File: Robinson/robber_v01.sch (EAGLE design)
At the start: 35 parts, among them J1 3.7_LIPO, J2 3.3-4.5 Motor, Q1 DMP1045U, Q2 MMBT2222A, U2 MCP73831

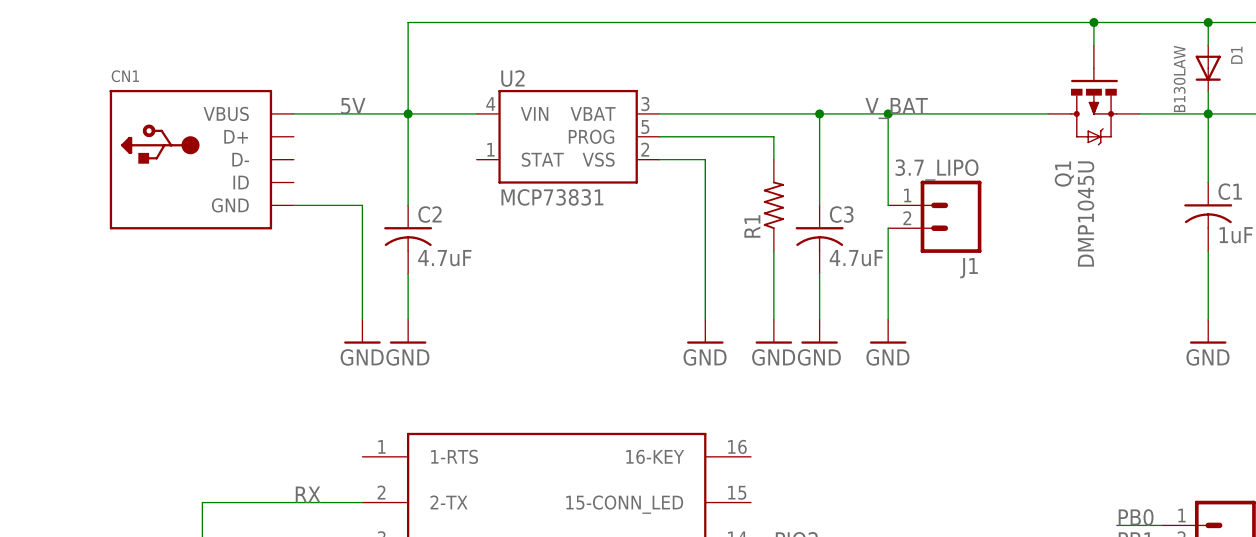
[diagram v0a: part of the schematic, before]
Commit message: ROBBER V01
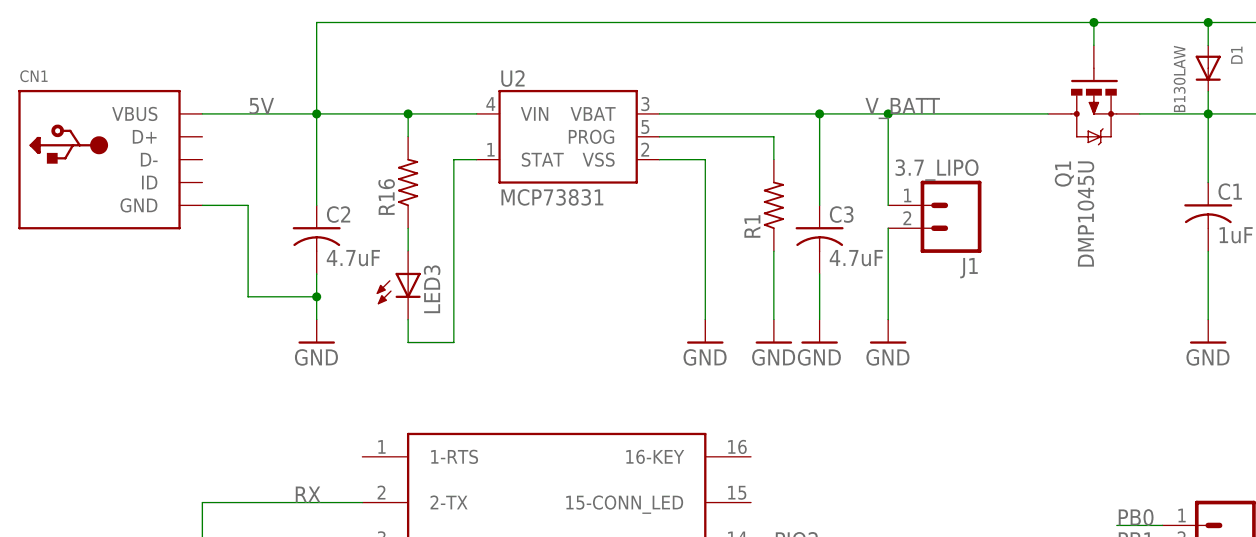
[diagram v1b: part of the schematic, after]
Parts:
- added LED3: (no value), led:LEDSML0603
- added R16: (no value), resistor:R-US_R0805
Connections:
- removed net V_BAT: C3.1, J1.1, Q1.D, U2.VBAT
- new net N$1: LED3.A, R16.1
- new net N$2: LED3.C, U2.STAT
- net 5V: now also R16.2
- net V_BATT: now also C3.1, J1.1, Q1.D, U2.VBAT
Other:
- moved on the sheet: C2, CN1
